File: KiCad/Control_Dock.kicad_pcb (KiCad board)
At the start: 2 copper layers, 137.9 x 68 mm, 22 parts, among them SW1 SW_Nidec_CAS-120A1, SW2 SW_Push, SW3 SW_Push, SW4 SW_Push

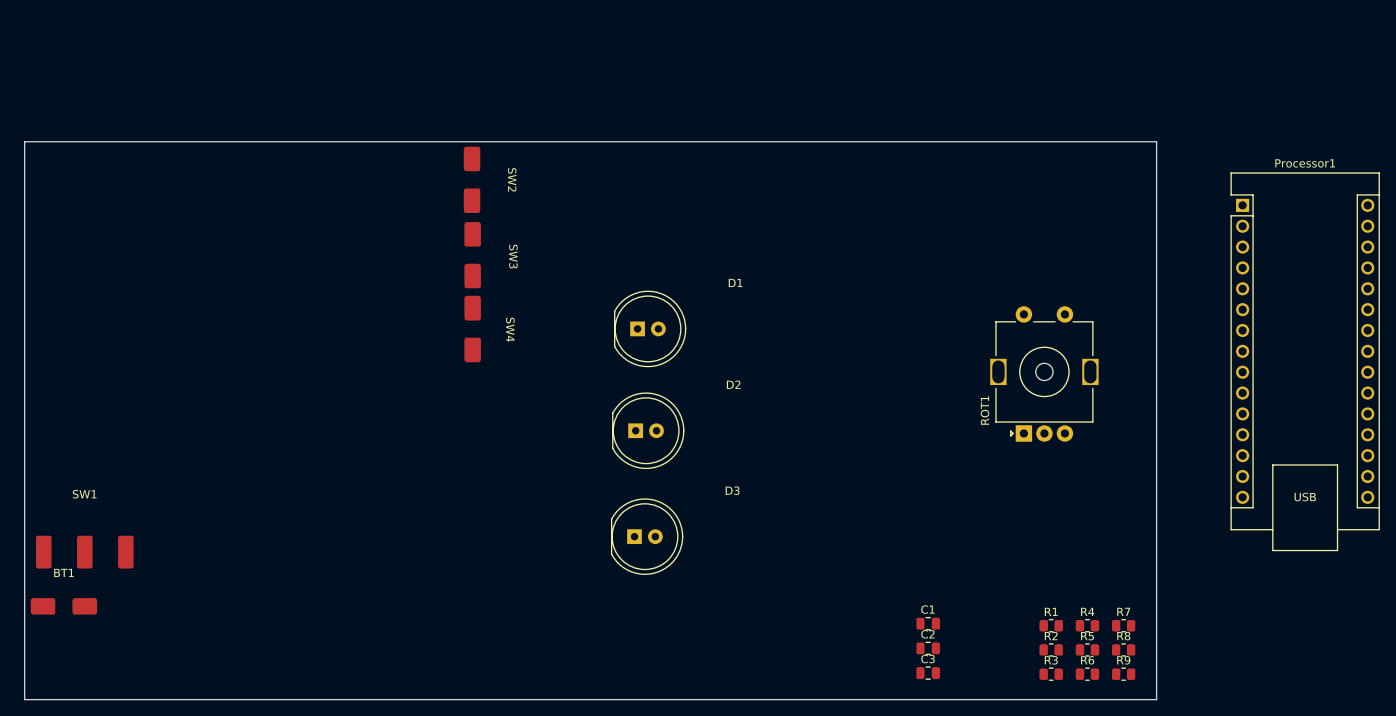
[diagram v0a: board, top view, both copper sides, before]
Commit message: Control PCB ready for review
Ready for review, then send to manufacturer
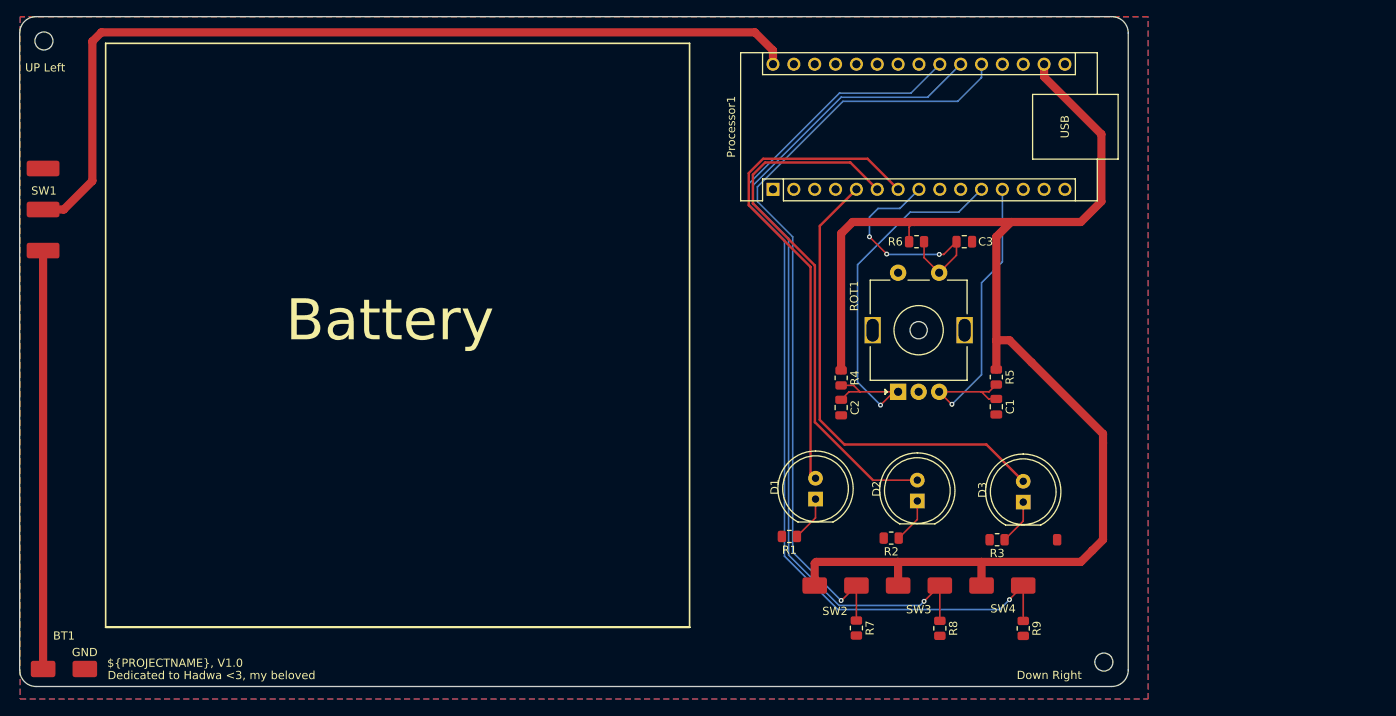
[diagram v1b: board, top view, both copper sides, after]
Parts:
- added Down Right: MountingHole_2.2mm_M2, MountingHole:MountingHole_2.2mm_M2, F.Cu at (180.0, 128.7)
- added UP Left: MountingHole_2.2mm_M2, MountingHole:MountingHole_2.2mm_M2, F.Cu at (50.9, 53.0)
- moved SW4 71.7 mm to (167.6, 119.4), turned to 0 degrees
- moved SW3 67.6 mm to (157.5, 119.4), turned to 0 degrees
- moved SW2 66.3 mm to (147.3, 119.4), turned to 0 degrees
- moved Processor1 57.2 mm to (139.7, 71.1), turned to 90 degrees
- moved R6 56.6 mm to (157.2, 77.5)
- moved C3 52.7 mm to (163.0, 77.5)
- moved D3 47.5 mm to (170.2, 109.2), turned to 90 degrees
- moved R4 42.6 mm to (148.0, 94.1), turned to -90 degrees
- moved SW1 41.2 mm to (49.8, 73.6), turned to 90 degrees
- moved D2 35.4 mm to (157.3, 109.1), turned to 90 degrees
- moved R5 35.0 mm to (166.9, 94.0), turned to -90 degrees
- moved R1 33.7 mm to (141.7, 113.4), turned to 180 degrees
- moved R7 32.6 mm to (149.9, 124.6), turned to -90 degrees
- moved C2 31.2 mm to (148.0, 97.7), turned to -90 degrees
- moved D1 30.0 mm to (144.9, 108.8), turned to 90 degrees
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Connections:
- BT1 pad 2: Net-(BT1--) -> GND
- SW1 pad 3: Net-(BT1--) -> GND
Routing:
- net +3.3V: track 0.00 -> 166.4 mm
- net /a3: track 0.00 -> 113.7 mm, vias 0 -> 1
- net +12V: track 0.00 -> 110.4 mm
- net /a2: track 0.00 -> 104.5 mm, vias 0 -> 1
- net /a1: track 0.00 -> 95.9 mm, vias 0 -> 1
- net /L2: track 0.00 -> 65.8 mm
- net /L3: track 0.00 -> 61.0 mm
- net /L1: track 0.00 -> 57.8 mm
- net Net-(BT1-+): track 0.00 -> 51.0 mm
- net ROT1_A: track 0.00 -> 49.9 mm, vias 0 -> 1
- net ROT1_B: track 0.00 -> 40.5 mm, vias 0 -> 1
- net ROT1_Sw: track 0.00 -> 31.2 mm, vias 0 -> 3
- net Net-(D3-K): track 0.00 -> 5.52 mm
- net Net-(D1-K): track 0.00 -> 5.49 mm
- net Net-(D2-K): track 0.00 -> 5.46 mm
- added copper zone on B.Cu, net GND
- added copper zone on F.Cu, net GND
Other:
- board size 137.9 x 68 mm -> 135 x 81.6 mm
- board text added: "${PROJECTNAME}, V${REVISION}"
- board text added: "Battery"
- board text added: "Dedicated to Hadwa <3, my beloved"
- board text added: "GND"
